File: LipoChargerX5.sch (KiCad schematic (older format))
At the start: 35 parts

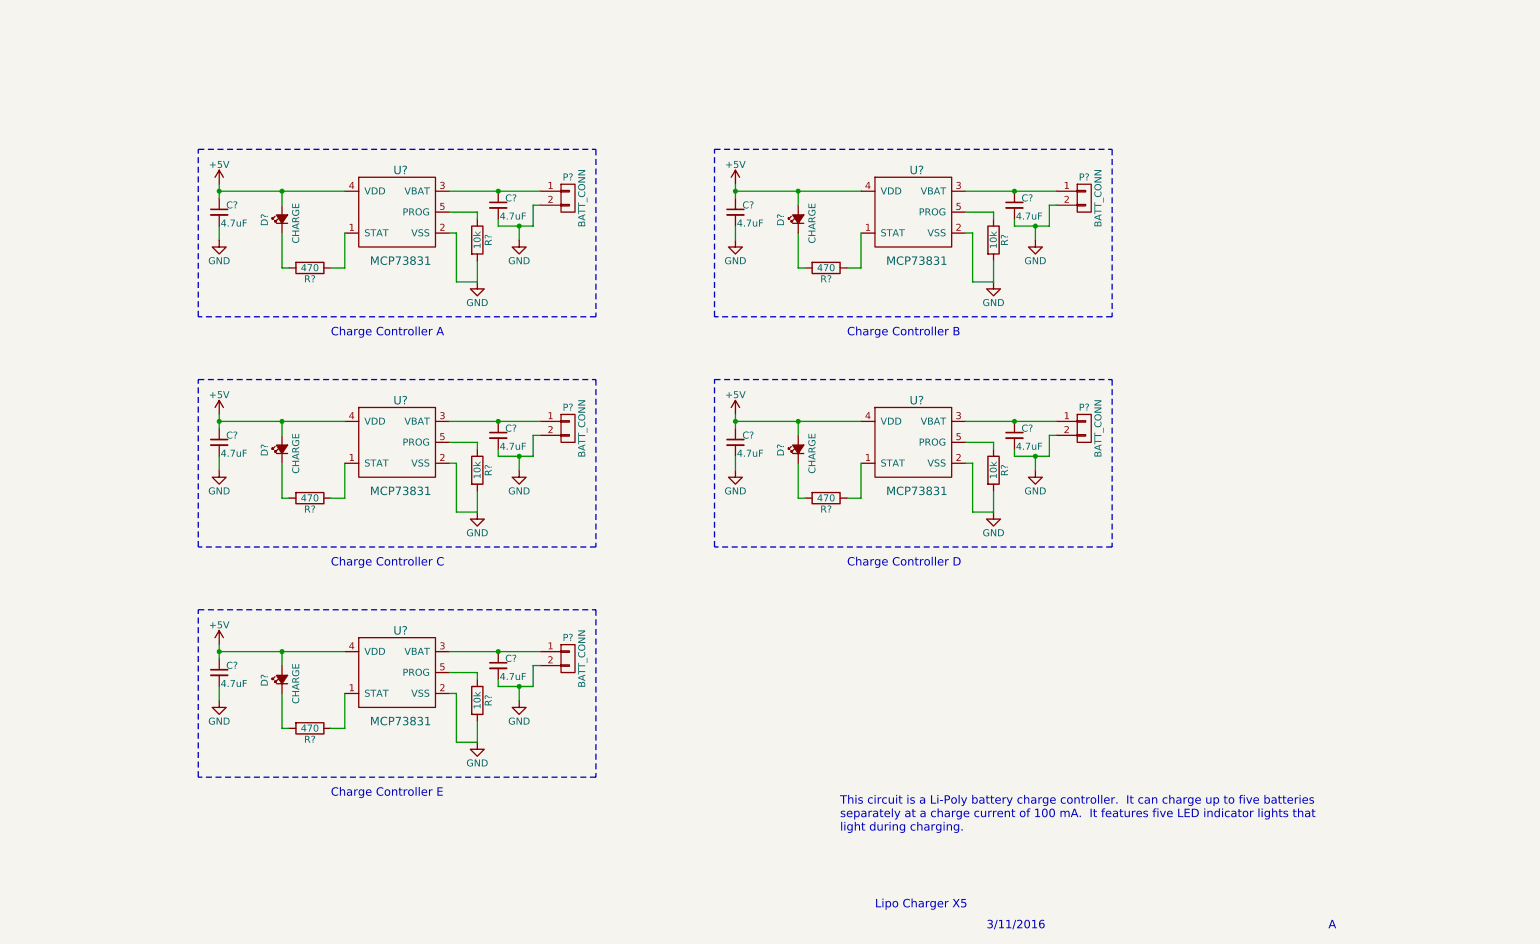
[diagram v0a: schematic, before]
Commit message: Finished Rev. A schematic
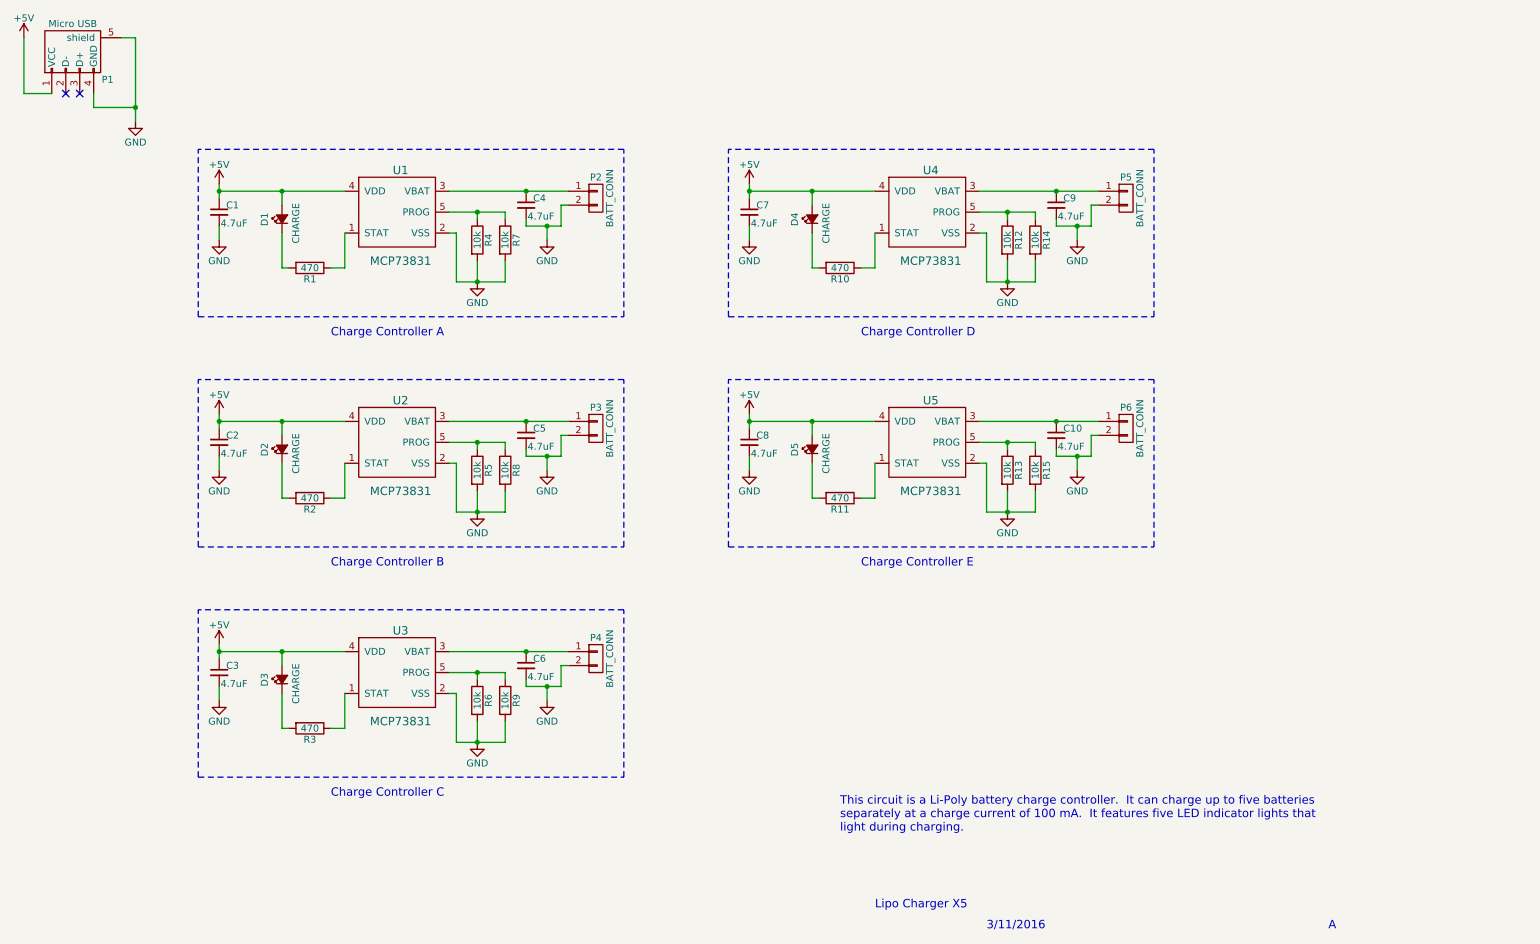
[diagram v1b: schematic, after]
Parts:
- removed C? (x8): 4.7uF, symbol C_Small
- removed D? (x4): CHARGE, symbol Led_Small
- removed P? (x4): BATT_CONN, symbol CONN_01X02
- removed R? (x4): 10k, symbol R
- removed R? (x4): 470, symbol R
- removed U? (x4): MCP73831, TO_SOT_Packages_SMD:SOT-23-5, symbol MCP73831
- added C10, C2, C3, C5, C6, C7, C8, C9: 4.7uF, symbol C_Small
- added D2, D3, D4, D5: CHARGE, symbol Led_Small
- added P1: Micro USB, symbol USB_B
- added P3, P4, P5, P6: BATT_CONN, symbol CONN_01X02
- added R10, R11, R2, R3: 470, symbol R
- added R12, R13, R14, R15, R5, R6, R7, R8, R9: 10k, symbol R
- added U2, U3, U4, U5: MCP73831, TO_SOT_Packages_SMD:SOT-23-5, symbol MCP73831
- gave numbers to parts that had none: 7
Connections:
- net +5V: now also C2.1, C3.1, C7.1, C8.1, D2.2 (A), D3.2 (A), D4.2 (A), D5.2 (A), P1.1 (VCC), U2.4 (VDD), U3.4 (VDD), U4.4 (VDD), U5.4 (VDD)
- net GND: now also C10.2, C2.2, C3.2, C5.2, C6.2, C7.2, C8.2, C9.2, P1.4 (GND), P1.5 (shield), P3.2 (P2), P4.2 (P2), P5.2 (P2), P6.2 (P2), R12.2, R13.2, R14.2, R15.2, R5.2, R6.2, R7.2, R8.2, R9.2, U2.2 (VSS), U3.2 (VSS), U4.2 (VSS), U5.2 (VSS)
- net at R4.1, U1.5 (PROG): now also R7.1
- new net: R10.1, U4.1 (STAT)
- new net: C9.1, P5.1 (P1), U4.3 (VBAT)
- new net: R12.1, R14.1, U4.5 (PROG)
- new net: D4.1 (K), R10.2
- new net: R2.1, U2.1 (STAT)
- new net: C5.1, P3.1 (P1), U2.3 (VBAT)
- new net: R5.1, R8.1, U2.5 (PROG)
- new net: D2.1 (K), R2.2
- new net: R11.1, U5.1 (STAT)
- new net: C10.1, P6.1 (P1), U5.3 (VBAT)
- new net: R13.1, R15.1, U5.5 (PROG)
- new net: D5.1 (K), R11.2
- new net: R3.1, U3.1 (STAT)
- new net: C6.1, P4.1 (P1), U3.3 (VBAT)
- new net: R6.1, R9.1, U3.5 (PROG)
- new net: D3.1 (K), R3.2
- no-connect marks 0 -> 2
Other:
- moved on the sheet: C4, P2

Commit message: Created connector footprint.  Associated components.  Began PCB layout.
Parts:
- C1, C10, C2, C3, C4, C5, C6, C7, C8, C9: footprint (none) -> Capacitors_SMD:C_0805
- D1, D2, D3, D4, D5: footprint (none) -> LEDs:LED_0805
- P1: footprint (none) -> Miscellanious:SMT-Micro-USB-AB
- P2, P3, P4, P5, P6: footprint (none) -> Connectors-Custom2:Eachine-Battery-Conn
- R1, R10, R11, R12, R13, R14, R15, R2, R3, R4, R5, R6, R7, R8, R9: footprint (none) -> Resistors_SMD:R_0805
